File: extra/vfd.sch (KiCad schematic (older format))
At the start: 25 parts

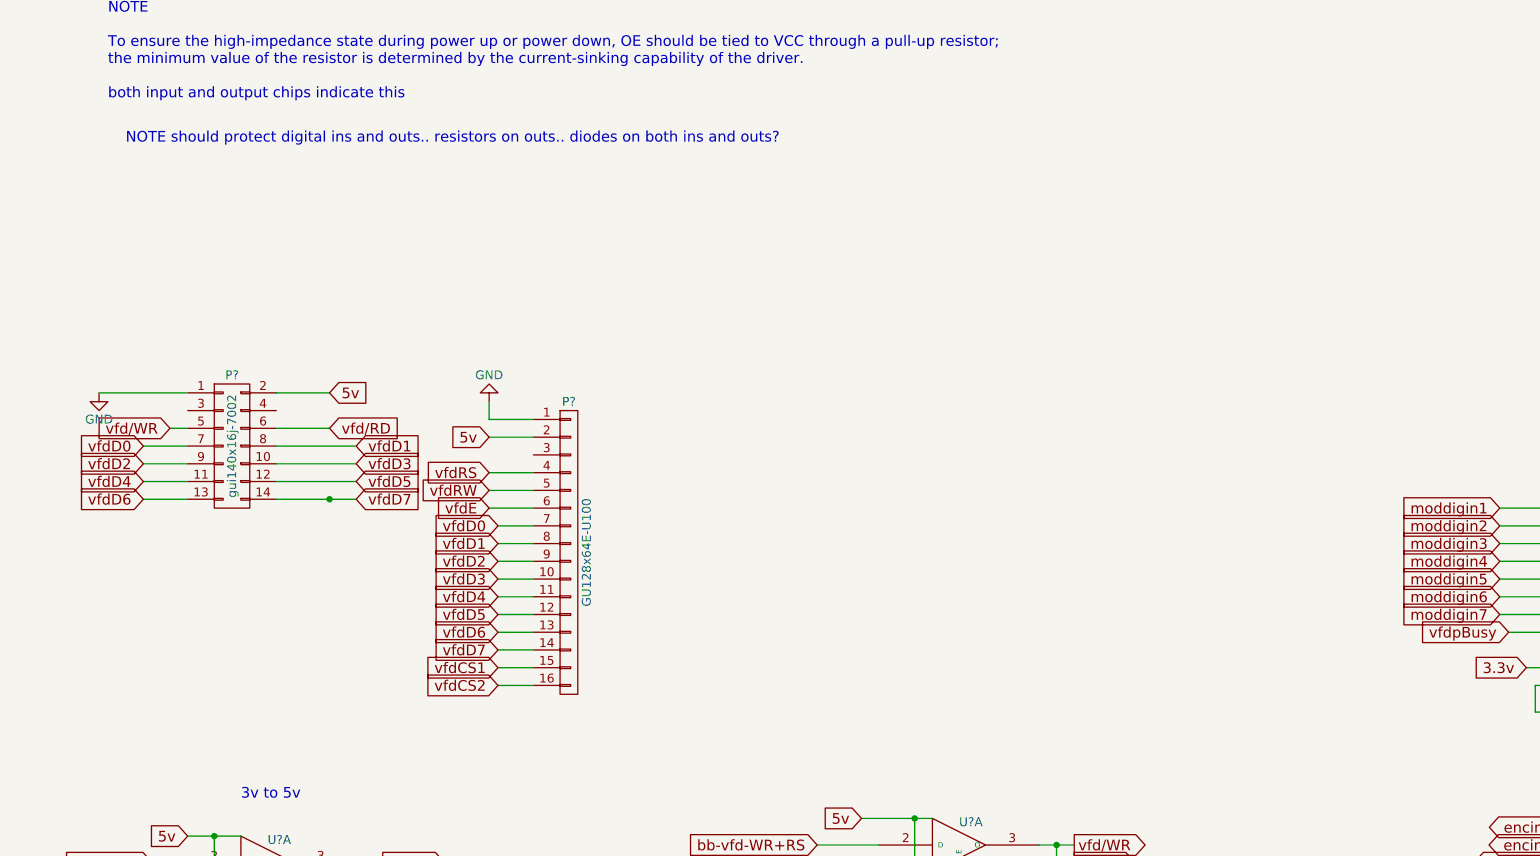
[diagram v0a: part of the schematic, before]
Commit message: a bunch more hooking up
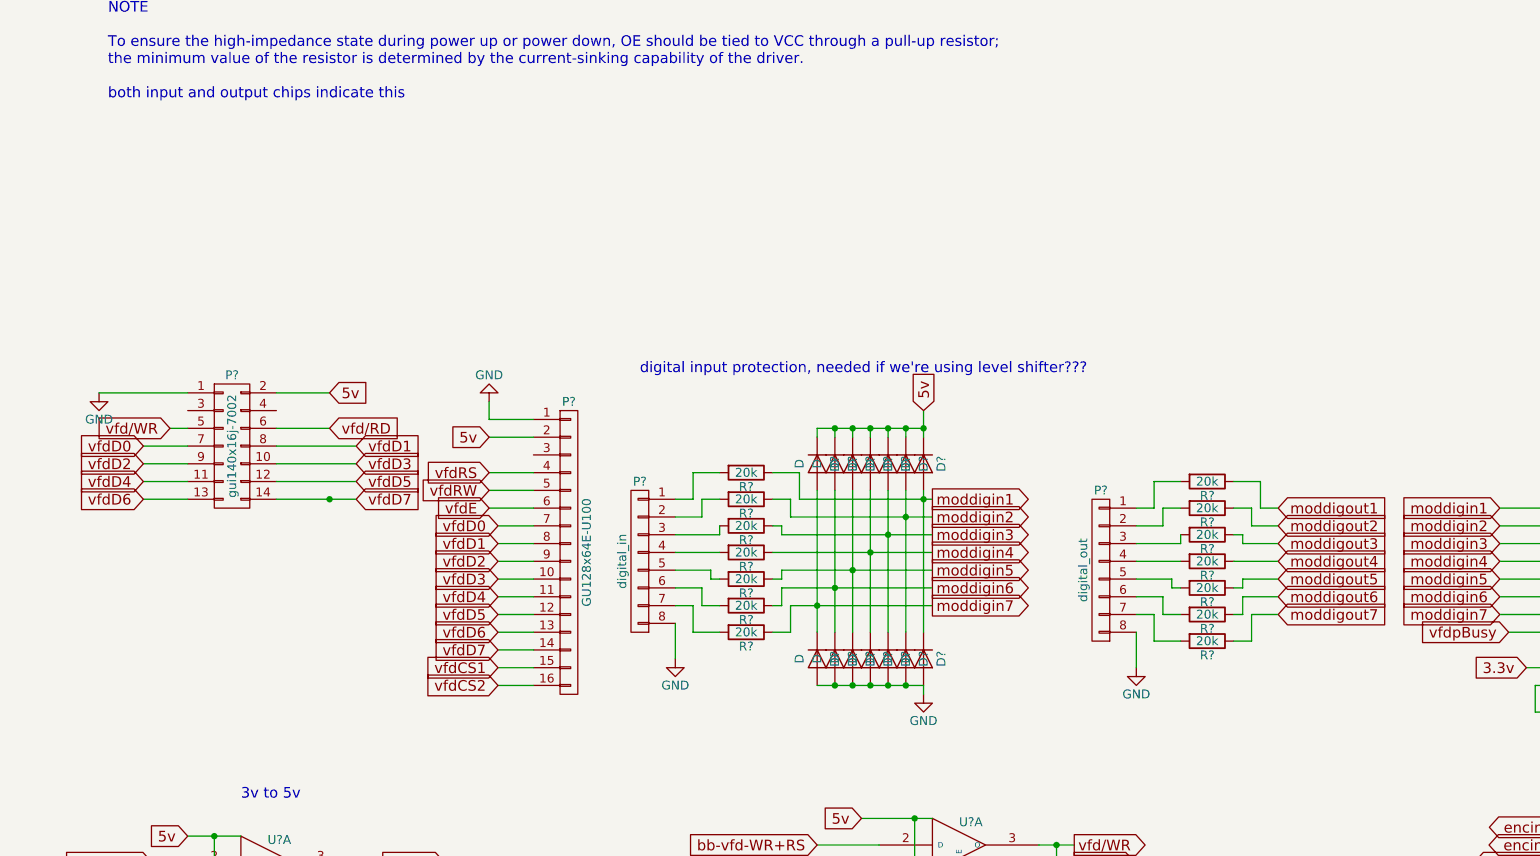
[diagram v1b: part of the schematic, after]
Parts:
- added D? (x14): D, symbol D
- added P?: digital_in, symbol CONN_01X08
- added P?: digital_out, symbol CONN_01X08
- added R? (x14): 20k, symbol R
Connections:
- net GND: now also D?.2 (A), D?.2 (A), D?.2 (A), D?.2 (A), D?.2 (A), D?.2 (A), D?.2 (A), P?.8 (P8), P?.8 (P8)
- net VCC: now also D?.1 (K), D?.1 (K), D?.1 (K), D?.1 (K), D?.1 (K), D?.1 (K), D?.1 (K)
- net moddigin1: now also D?.1 (K), D?.2 (A), R?.1
- net moddigin2: now also D?.1 (K), D?.2 (A), R?.1
- net moddigin3: now also D?.1 (K), D?.2 (A), R?.1
- net moddigin4: now also D?.1 (K), D?.2 (A), R?.1
- net moddigin5: now also D?.1 (K), D?.2 (A), R?.1
- net moddigin6: now also D?.1 (K), D?.2 (A), R?.1
- net moddigin7: now also D?.1 (K), D?.2 (A), R?.1
- net moddigout1: now also R?.1
- net moddigout2: now also R?.1
- net moddigout3: now also R?.1
- net moddigout4: now also R?.1
- net moddigout5: now also R?.1
- net moddigout6: now also R?.1
- net moddigout7: now also R?.1
- new net: P?.1 (P1), R?.2 (x2)
- new net: P?.2 (P2), R?.2 (x2)
- new net: P?.3 (P3), R?.2 (x2)
- new net: P?.4 (P4), R?.2 (x2)
- new net: P?.5 (P5), R?.2 (x2)
- new net: P?.6 (P6), R?.2 (x2)
- new net: P?.7 (P7), R?.2 (x2)
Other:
- note added: "digital input protection, needed if we're using level shifter???"
- note removed: "NOTE should protect digital ins and outs.. resistors on outs.. diodes on both ins and outs?"
